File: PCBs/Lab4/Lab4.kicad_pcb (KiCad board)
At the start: 2 copper layers, 13 parts, among them IC1 M0C1103QDDFRQ1, J1 Conn_01x05_Pin, SW1 SW_SPST, SW2 SW_SPST

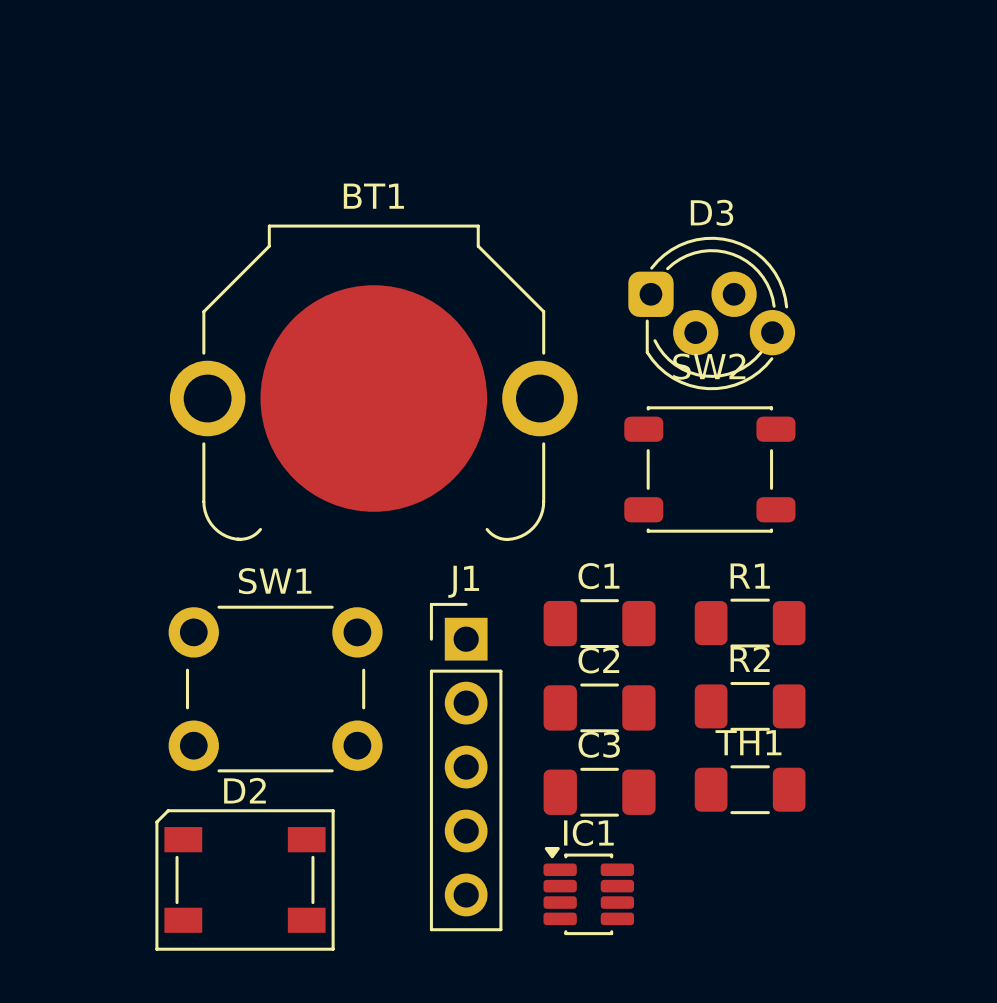
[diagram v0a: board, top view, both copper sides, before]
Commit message: update
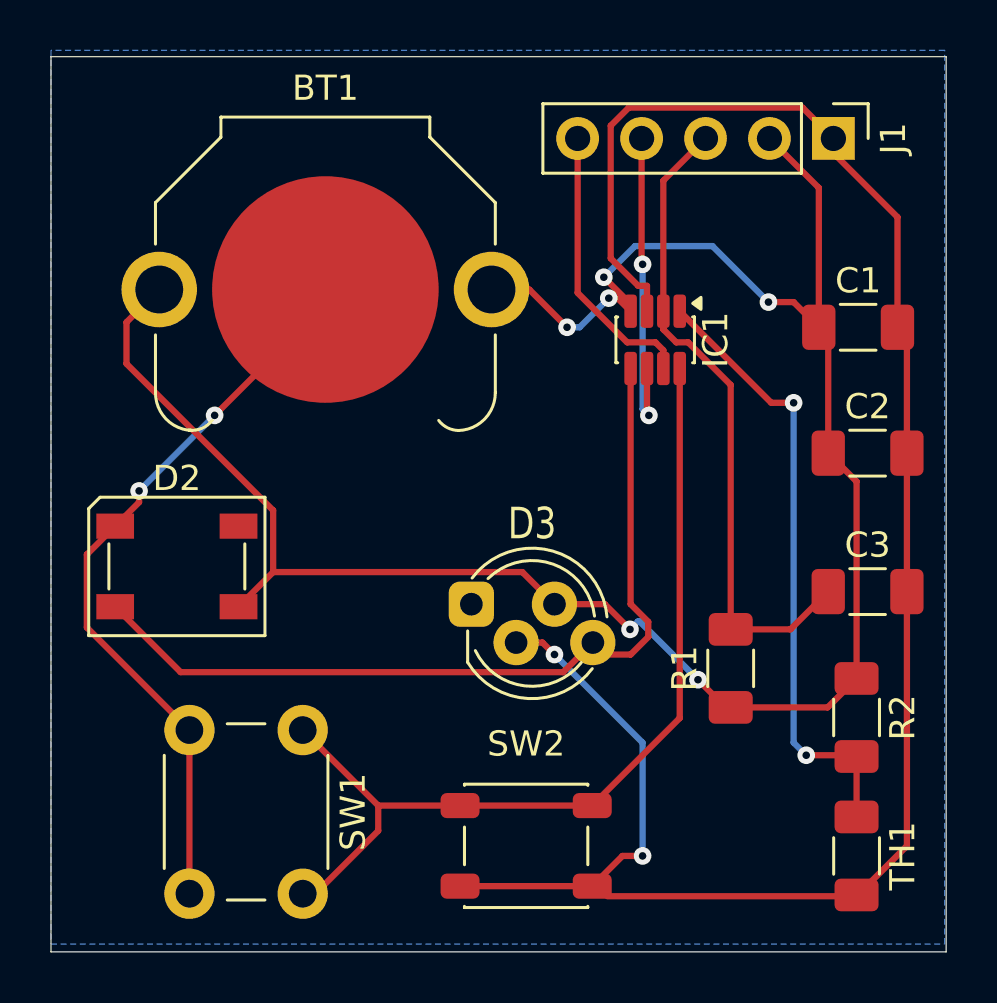
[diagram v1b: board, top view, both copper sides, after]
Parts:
- J1: value Conn_01x05_Pin -> Conn
- moved J1 24.7 mm to (158.1, 82.5), turned to -90 degrees
- moved IC1 22.2 mm to (151.0, 90.5), turned to -90 degrees
- moved SW2 16.6 mm to (145.9, 110.6)
- moved C1 15.6 mm to (159.1, 90.0)
- moved C2 14.7 mm to (159.4, 95.0)
- moved D3 14.2 mm to (143.7, 101.0)
- moved C3 13.3 mm to (159.4, 100.5)
- moved D2 12.7 mm to (132.0, 99.5)
- moved SW1 5.81 mm to (137.0, 106.0), turned to -90 degrees
- moved TH1 4.98 mm to (159.0, 111.0), turned to -90 degrees
- moved BT1 4.74 mm to (137.9, 88.5)
- moved R2 4.25 mm to (159.0, 105.5), turned to -90 degrees
- moved R1 1.96 mm to (154.0, 103.5), turned to 90 degrees
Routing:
- net GND: track 0.00 -> 107.4 mm, vias 0 -> 4
- net VDD: track 0.00 -> 84.2 mm, vias 0 -> 6
- net Button: track 0.00 -> 36.6 mm
- net LED_DIN: track 0.00 -> 34.8 mm
- net NRST: track 0.00 -> 26.1 mm
- net THRM: track 0.00 -> 24.7 mm, vias 0 -> 2
- net SWDIO: track 0.00 -> 13.6 mm, vias 0 -> 2
- net SWCLK: track 0.00 -> 11.2 mm
- added copper zone on B.Cu, net GND
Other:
- board outline added: 35.6 x 35.6 mm
- board text added: "Battery_Cell"
- board text added: "D.V."
